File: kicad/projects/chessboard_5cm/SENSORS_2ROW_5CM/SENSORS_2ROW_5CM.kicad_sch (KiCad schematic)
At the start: 13 parts, among them J2 Conn_02x05_Odd_Even

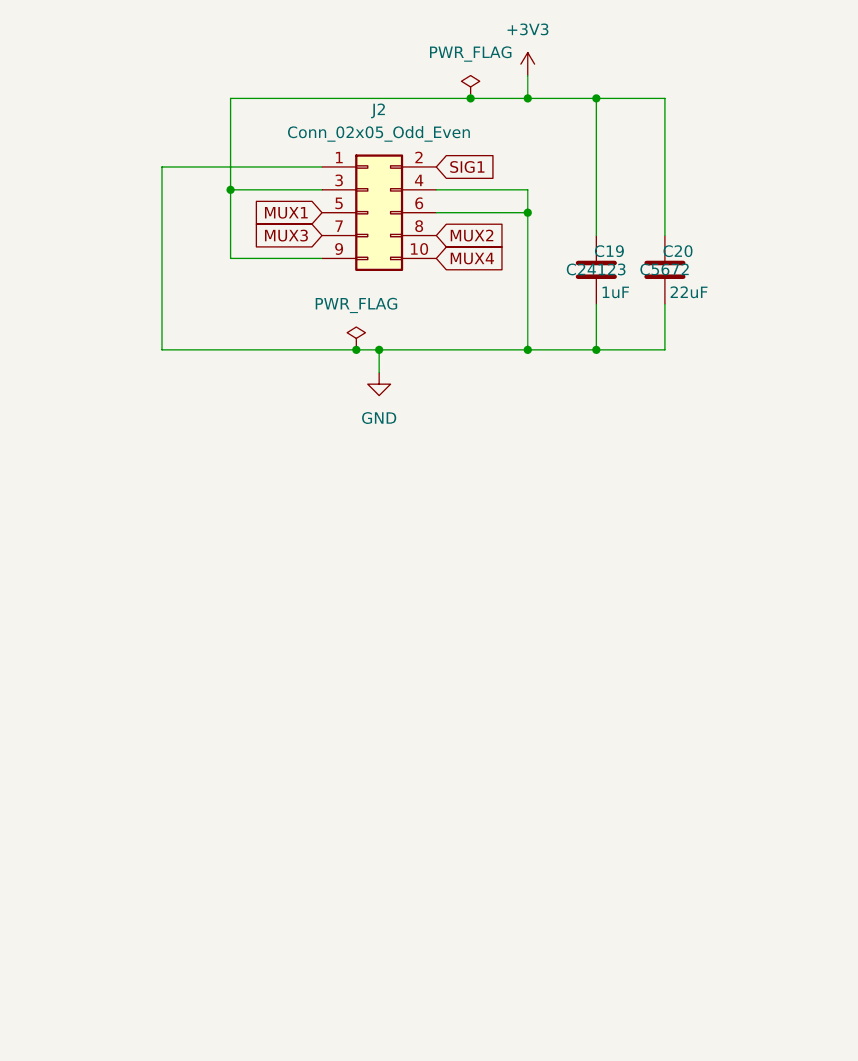
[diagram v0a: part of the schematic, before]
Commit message: interconnect 5cm finished. brain v2 with changes pending
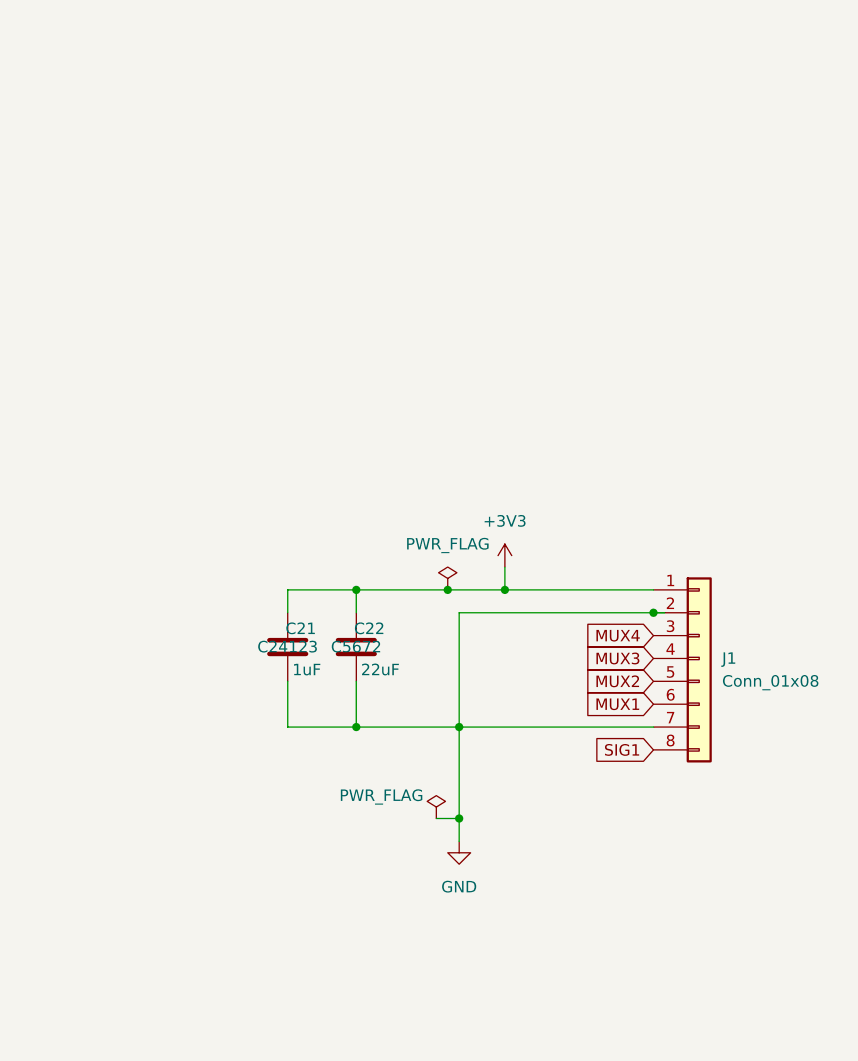
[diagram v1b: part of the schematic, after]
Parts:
- removed C19: 1uF, Capacitor_SMD:C_0805_2012Metric_Pad1.18x1.45mm_HandSolder, symbol Device:C
- removed C20: 22uF, Capacitor_SMD:C_1206_3216Metric_Pad1.33x1.80mm_HandSolder, symbol Device:C
- removed J2: Conn_02x05_Odd_Even, Connector_PinHeader_2.54mm:PinHeader_2x05_P2.54mm_Vertical, symbol Connector_Generic:Conn_02x05_Odd_Even
- added C21: 1uF, Capacitor_SMD:C_0805_2012Metric_Pad1.18x1.45mm_HandSolder, symbol Device:C
- added C22: 22uF, Capacitor_SMD:C_1206_3216Metric_Pad1.33x1.80mm_HandSolder, symbol Device:C
- added J1: Conn_01x08, Connector_PinHeader_2.54mm:PinHeader_1x08_P2.54mm_Horizontal, symbol Connector_Generic:Conn_01x08
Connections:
- net +3V3: now also C21.1, C22.1, J1.1 (Pin_1)
- net GND: now also C21.2, C22.2, J1.2 (Pin_2), J1.7 (Pin_7)
- net MUX1: now also J1.6 (Pin_6)
- net MUX2: now also J1.5 (Pin_5)
- net MUX3: now also J1.4 (Pin_4)
- net MUX4: now also J1.3 (Pin_3)
- net SIG1: now also J1.8 (Pin_8)

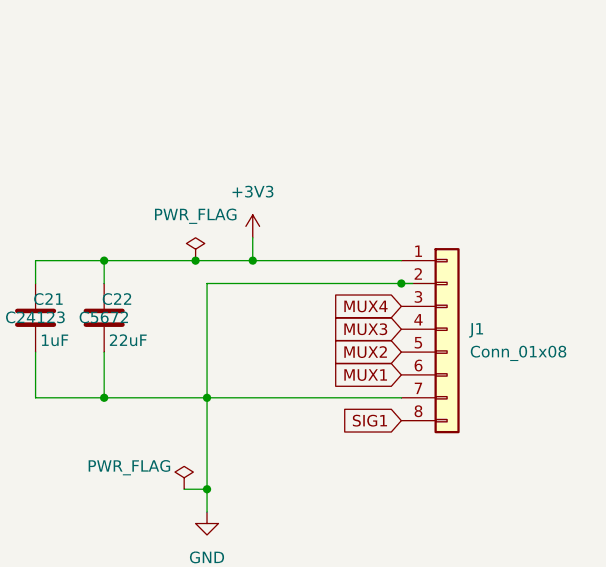
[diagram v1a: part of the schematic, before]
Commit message: ready for manufacturing
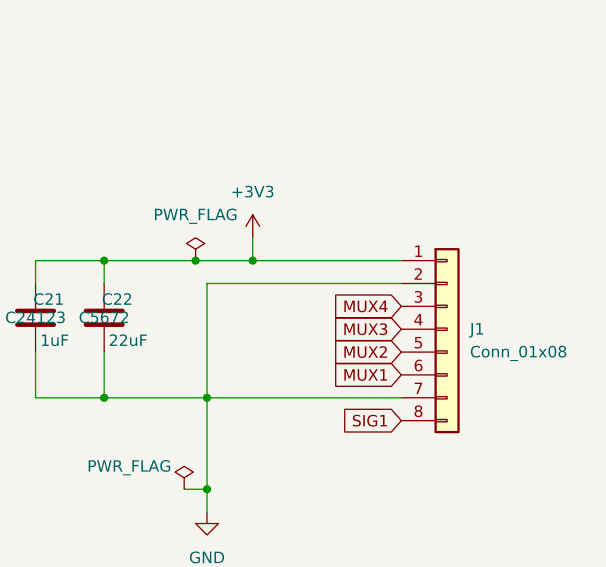
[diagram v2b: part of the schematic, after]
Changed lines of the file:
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@@
-	)
-	(junction
-		(at 223.52 104.14)
-		(diameter 0)
-		(color 0 0 0 0)
 	)
 	(junction
@@
 	(wire
 		(pts
+			(xy 223.52 104.14) (xy 201.93 104.14)
+		)
+		(stroke
+			(width 0)
+			(type default)
+		)
+	)
+	(wire
+		(pts
 			(xy 182.88 101.6) (xy 182.88 104.14)
 		)
@@
 	(wire
 		(pts
-			(xy 223.52 104.14) (xy 201.93 104.14)
-		)
-		(stroke
-			(width 0)
-			(type default)
-		)
-	)
-	(wire
-		(pts
 			(xy 77.47 140.97) (xy 77.47 138.43)
 		)
 		(stroke
-			(width 0)
-			(type default)
-		)
-	)
-	(wire
-		(pts
-			(xy 224.79 104.14) (xy 223.52 104.14)
-		)
-		(stroke
